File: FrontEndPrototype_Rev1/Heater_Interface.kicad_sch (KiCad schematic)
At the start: 10 parts, among them J19 Conn_01x02_Pin, J20 Conn_01x02_Pin, J21 Conn_01x02_Pin, J22 Conn_01x02_Pin, Q1 PMV30UN2

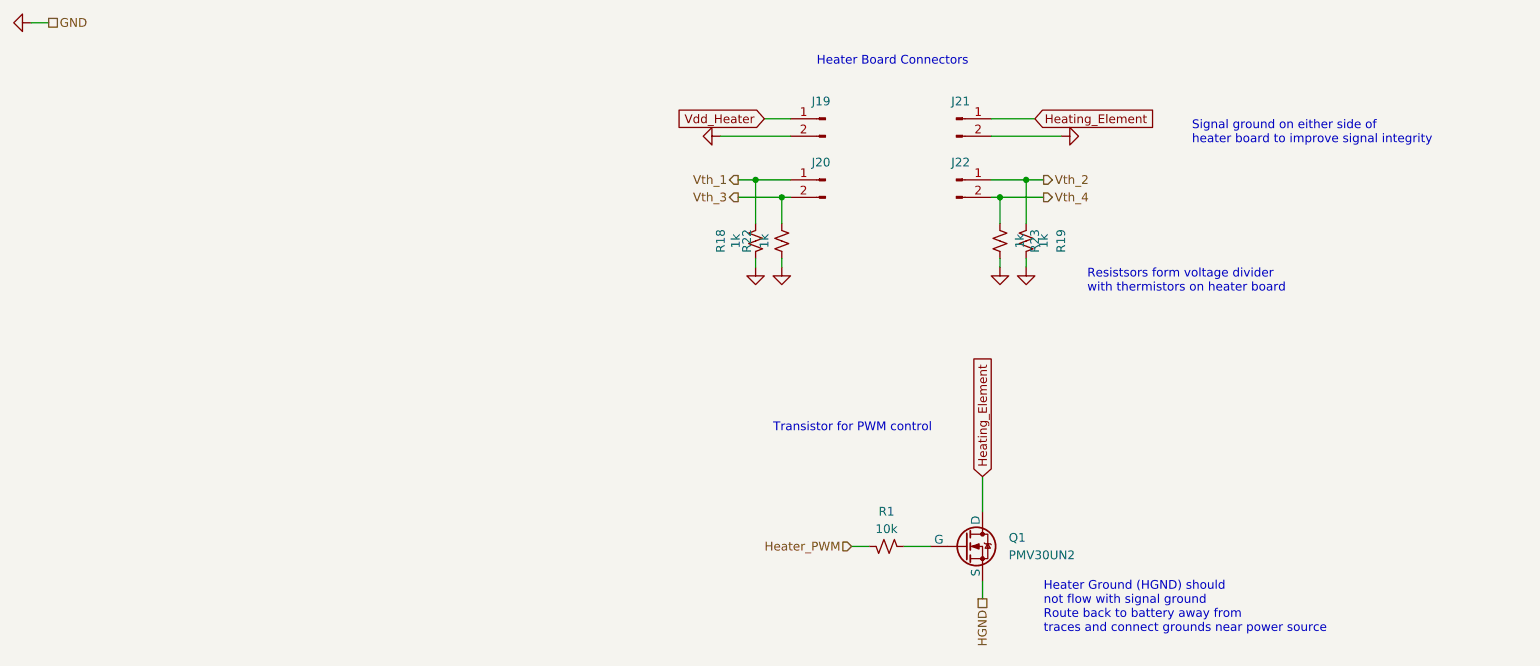
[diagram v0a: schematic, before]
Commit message: First Pass Schematic Fixes for Power Management Board
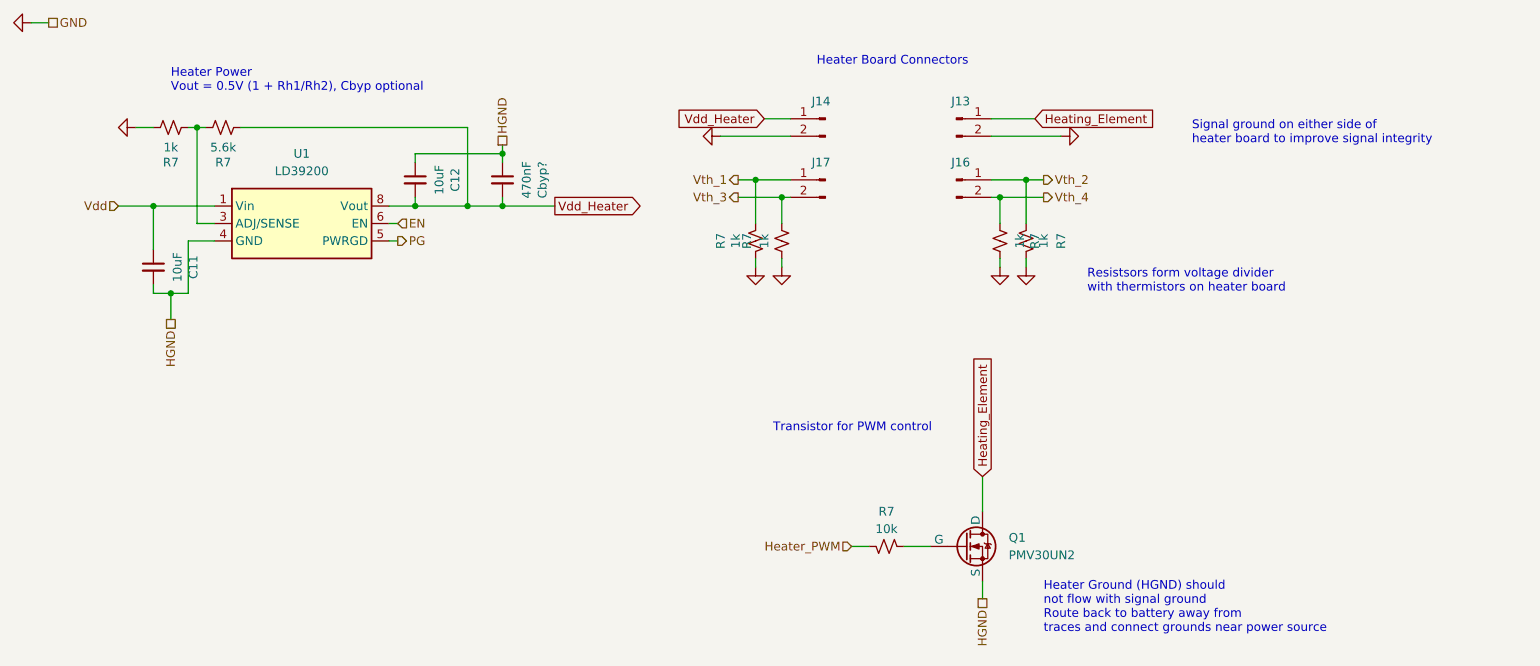
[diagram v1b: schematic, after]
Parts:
- added C11, C12: 10uF, Capacitor_SMD:C_0603_1608Metric_Pad1.08x0.95mm_HandSolder, symbol Device:C_Small
- added Cbyp?: 470nF, Capacitor_SMD:C_0603_1608Metric_Pad1.08x0.95mm_HandSolder, symbol Device:C_Small
- added R7: 5.6k, Resistor_SMD:R_0603_1608Metric_Pad0.98x0.95mm_HandSolder, symbol Device:R_Small_US
- added R7: 1k, Resistor_SMD:R_0603_1608Metric_Pad0.98x0.95mm_HandSolder, symbol Device:R_Small_US
- added U1: LD39200, Package_DFN_QFN:DFN-8-1EP_4x4mm_P0.8mm_EP2.3x3.24mm, symbol FrontEndPrototype_Rev1-rescue:LD39200
- renumbered J21 to J13, J19 to J14, J22 to J16, J20 to J17, R1 to R7, R23 to R7, R18 to R7, R22 to R7, R19 to R7
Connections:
- net GND: now also R7.1
- net HGND: now also C11.2, C12.1, Cbyp?.1, U1.4 (GND), U1.9 (GND)
- net Vdd_Heater: now also C12.2, Cbyp?.2, R7.2, U1.7 (Vout), U1.8 (Vout)
- new net: R7.1, R7.2, U1.3 (ADJ/SENSE)
- new net EN: U1.6 (EN)
- new net PG: U1.5 (PWRGD)
- new net Vdd: C11.1, U1.1 (Vin), U1.2 (Vin)
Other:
- note added: "Heater Power Vout = 0.5V (1 + Rh1/Rh2), Cbyp optional"

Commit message: Updated Measurement Board with new 3V Reference
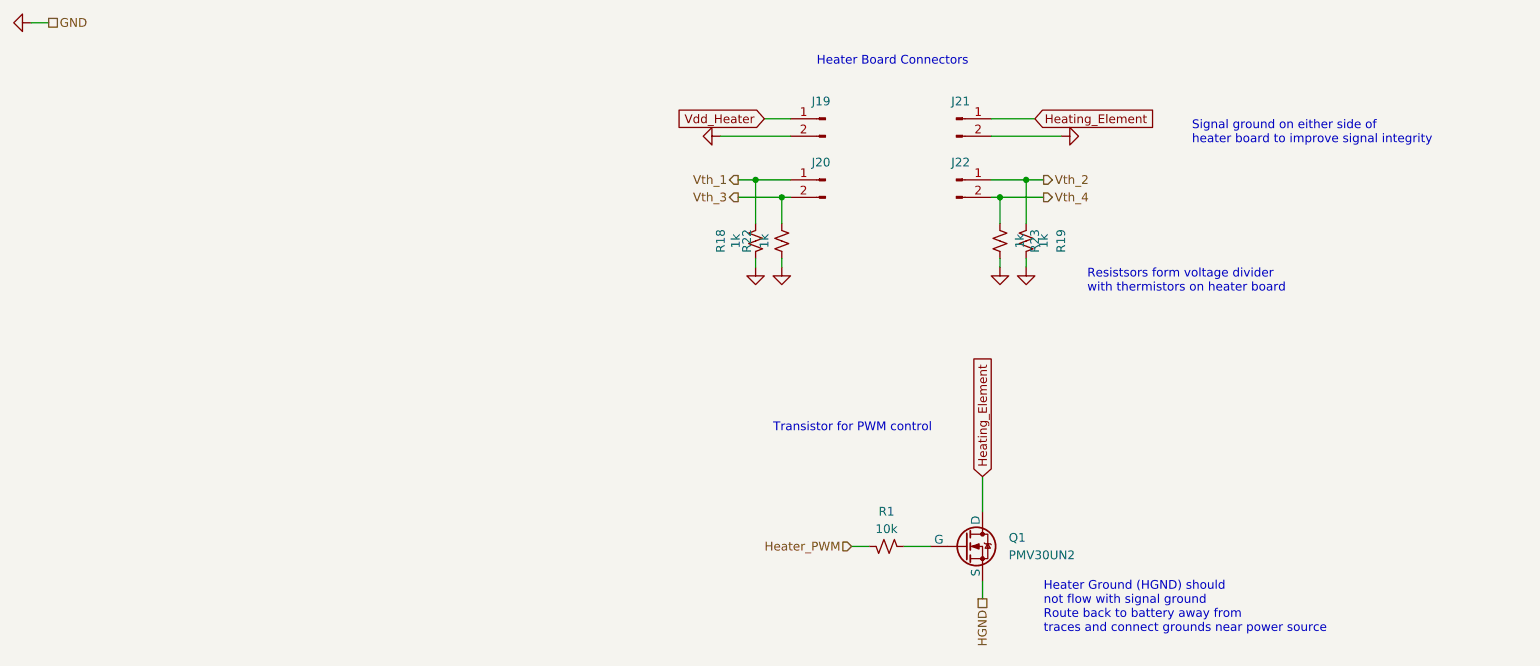
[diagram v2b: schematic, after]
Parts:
- removed C11, C12: 10uF, Capacitor_SMD:C_0603_1608Metric_Pad1.08x0.95mm_HandSolder, symbol Device:C_Small
- removed Cbyp?: 470nF, Capacitor_SMD:C_0603_1608Metric_Pad1.08x0.95mm_HandSolder, symbol Device:C_Small
- removed R7: 5.6k, Resistor_SMD:R_0603_1608Metric_Pad0.98x0.95mm_HandSolder, symbol Device:R_Small_US
- removed R7: 1k, Resistor_SMD:R_0603_1608Metric_Pad0.98x0.95mm_HandSolder, symbol Device:R_Small_US
- removed U1: LD39200, Package_DFN_QFN:DFN-8-1EP_4x4mm_P0.8mm_EP2.3x3.24mm, symbol FrontEndPrototype_Rev1-rescue:LD39200
- renumbered J14 to J19, J17 to J20, J13 to J21, J16 to J22, R7 to R1, R7 to R18, R7 to R19, R7 to R22, R7 to R23
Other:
- note removed: "Heater Power Vout = 0.5V (1 + Rh1/Rh2), Cbyp optional"
